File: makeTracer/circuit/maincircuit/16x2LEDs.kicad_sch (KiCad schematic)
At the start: 4 parts, among them P1 AirWirePort, P2 AirWirePort, U2 74HC595, U3 74HC595

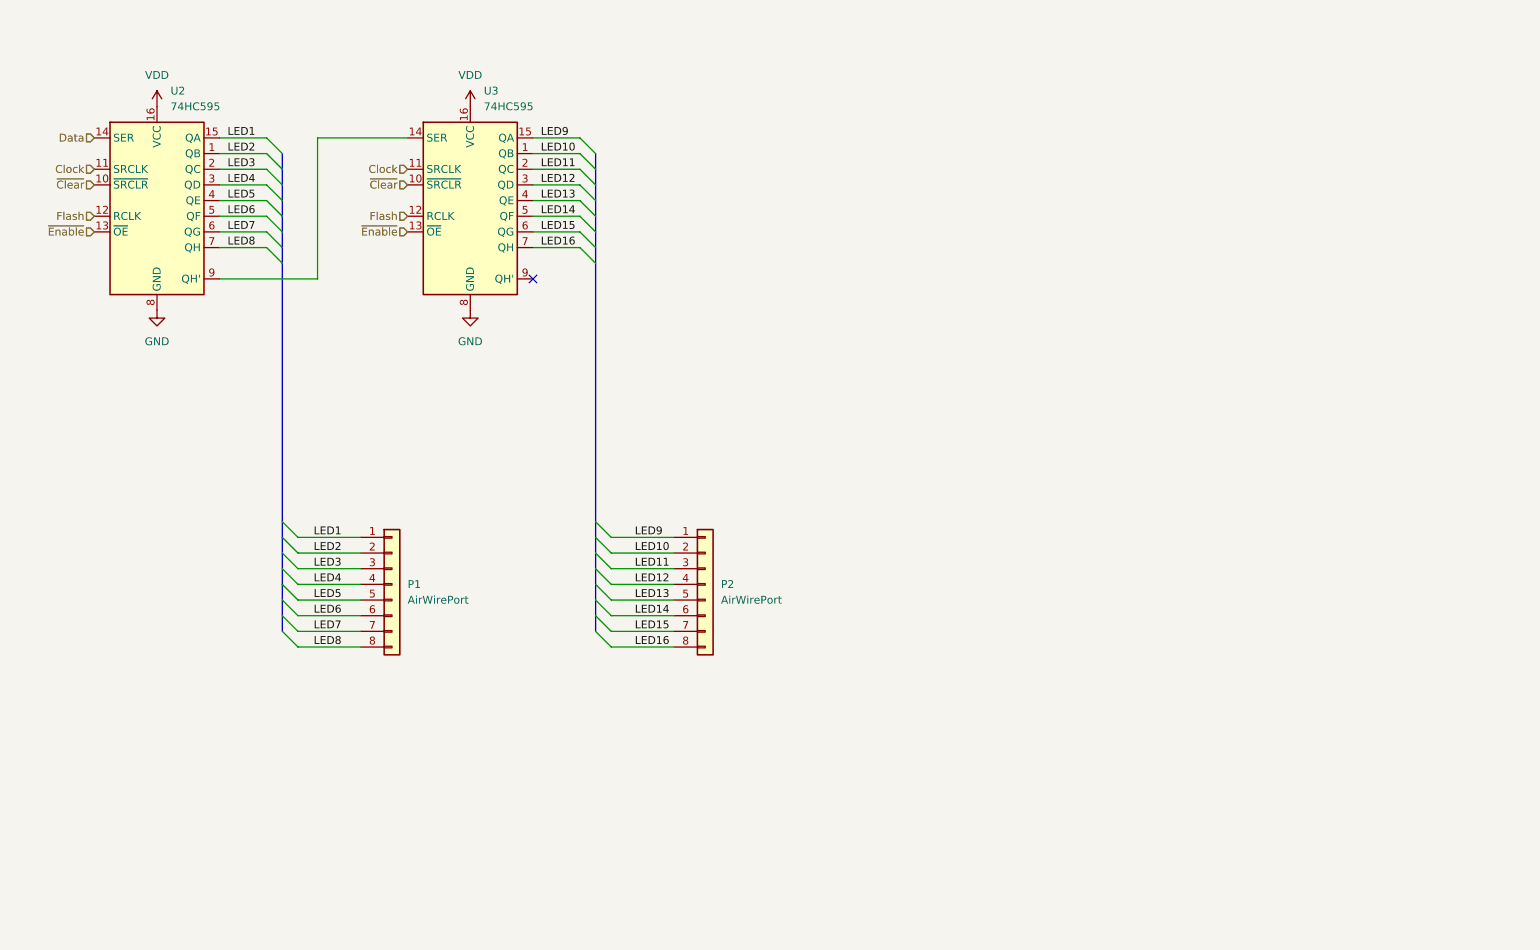
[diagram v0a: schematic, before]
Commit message: done: maincircuit
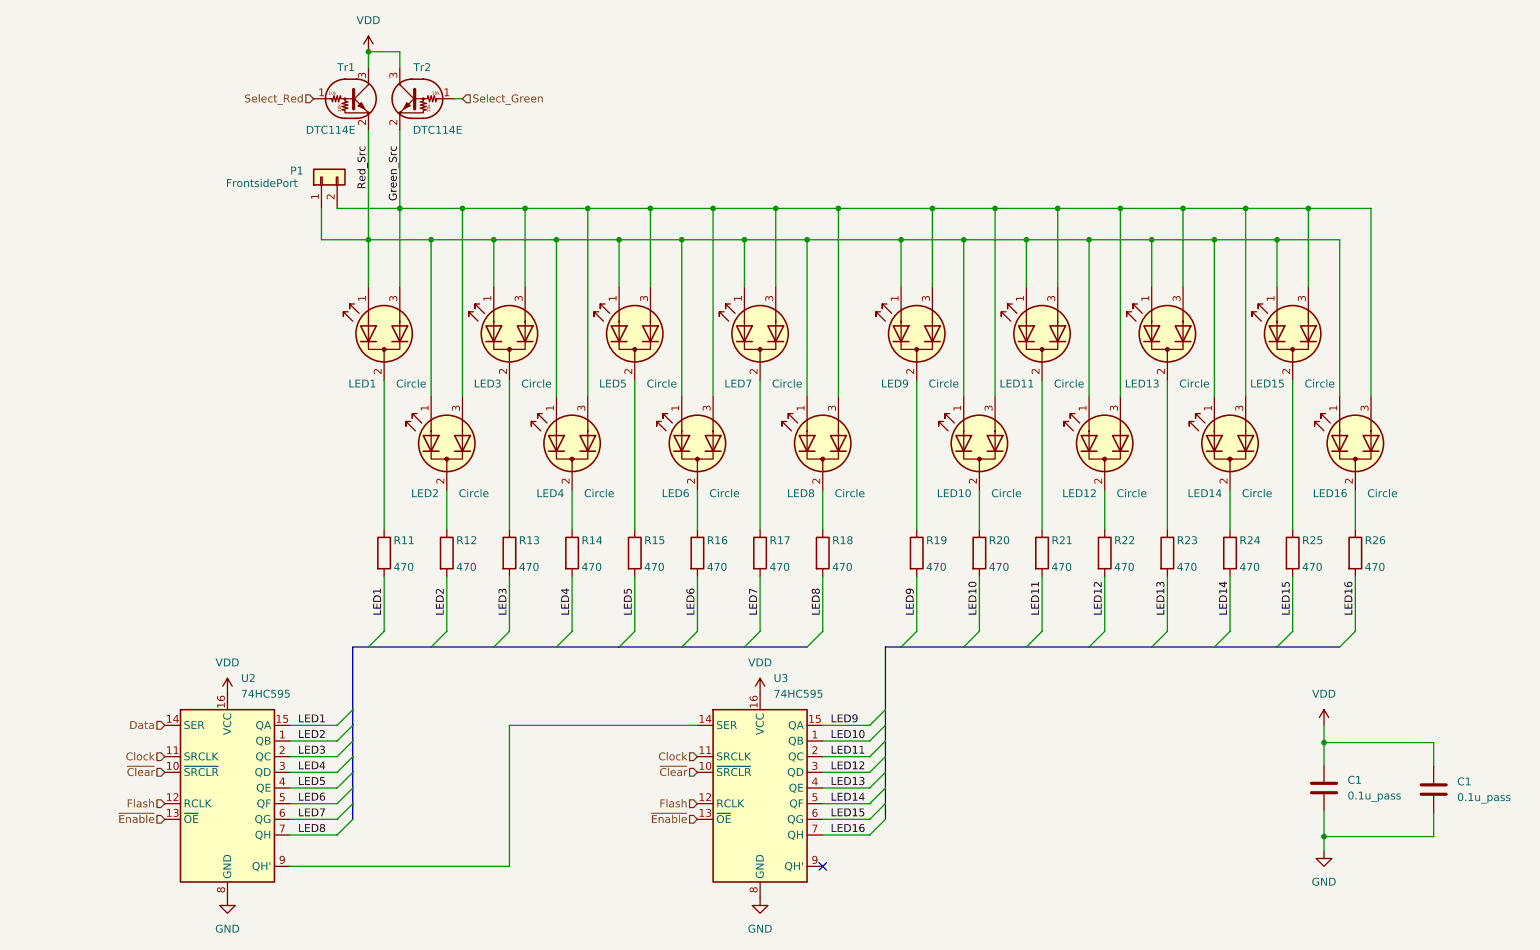
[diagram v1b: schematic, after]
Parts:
- removed P1, P2: AirWirePort, Connector_PinHeader_2.54mm:PinHeader_1x08_P2.54mm_Vertical, symbol Connector_Generic:Conn_01x08
- added C1 (x2): 0.1u_pass, Capacitor_THT:C_Disc_D5.0mm_W2.5mm_P2.50mm, symbol Device:C
- added LED1, LED10, LED11, LED12, LED13, LED14, LED15, LED16, LED2, LED3, LED4, LED5, LED6, LED7, LED8, LED9: Circle, LED_THT:LED_D3.0mm-3, symbol Device:LED_Dual_AKA
- added P1: FrontsidePort, Connector_PinHeader_2.54mm:PinHeader_1x02_P2.54mm_Vertical, symbol Connector_Generic:Conn_01x02
- added R11, R13, R14, R15, R16, R17, R18, R19, R20, R21, R22, R23, R24, R25, R26: 470, Resistor_THT:R_Axial_DIN0207_L6.3mm_D2.5mm_P2.54mm_Vertical, symbol Device:R
- added R12: 470, Resistor_THT:R_Axial_DIN0207_L6.3mm_D2.5mm_P15.24mm_Horizontal, symbol Device:R
- added Tr1, Tr2: DTC114E, Package_TO_SOT_THT:TO-92, symbol Transistor_BJT:DTC114E
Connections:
- net GND: now also C1.2, C1.2
- net LED1: now also R11.2
- net LED10: now also R20.2
- net LED11: now also R21.2
- net LED12: now also R22.2
- net LED13: now also R23.2
- net LED14: now also R24.2
- net LED15: now also R25.2
- net LED16: now also R26.2
- net LED2: now also R12.2
- net LED3: now also R13.2
- net LED4: now also R14.2
- net LED5: now also R15.2
- net LED6: now also R16.2
- net LED7: now also R17.2
- net LED8: now also R18.2
- net LED9: now also R19.2
- net VDD: now also C1.1, C1.1, Tr1.3 (C), Tr2.3 (C)
- new net: LED4.2 (K), R14.1
- new net: LED12.2 (K), R22.1
- new net: LED1.2 (K), R11.1
- new net: LED3.2 (K), R13.1
- new net: LED11.2 (K), R21.1
- new net: LED13.2 (K), R23.1
- new net: LED9.2 (K), R19.1
- new net: LED15.2 (K), R25.1
- new net: LED14.2 (K), R24.1
- new net: LED16.2 (K), R26.1
- new net: LED10.2 (K), R20.1
- new net: LED5.2 (K), R15.1
- new net: LED8.2 (K), R18.1
- new net: LED6.2 (K), R16.1
- new net: LED7.2 (K), R17.1
- new net: LED2.2 (K), R12.1
- new net Green_Src: LED1.3 (A2), LED10.3 (A2), LED11.3 (A2), LED12.3 (A2), LED13.3 (A2), LED14.3 (A2), LED15.3 (A2), LED16.3 (A2), LED2.3 (A2), LED3.3 (A2), LED4.3 (A2), LED5.3 (A2), LED6.3 (A2), LED7.3 (A2), LED8.3 (A2), LED9.3 (A2), P1.2 (Pin_2), Tr2.2 (E)
- new net Red_Src: LED1.1 (A1), LED10.1 (A1), LED11.1 (A1), LED12.1 (A1), LED13.1 (A1), LED14.1 (A1), LED15.1 (A1), LED16.1 (A1), LED2.1 (A1), LED3.1 (A1), LED4.1 (A1), LED5.1 (A1), LED6.1 (A1), LED7.1 (A1), LED8.1 (A1), LED9.1 (A1), P1.1 (Pin_1), Tr1.2 (E)
- new net Select_Green: Tr2.1 (B)
- new net Select_Red: Tr1.1 (B)
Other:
- moved on the sheet: U2, U3
